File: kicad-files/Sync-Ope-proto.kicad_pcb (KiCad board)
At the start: 2 copper layers, 100 x 100 mm, 66 parts, among them J1 rca, J10 rca, J2 europower, J3 mono_jack_3.5mm, J4 mono_jack_3.5mm, J5 mono_jack_3.5mm, J6 rca, J7 barrel_jack, J8 diy_power_header, J9 rca, U1 AD8072, U2 74HC4538, U3 L7805, U4 L7905, U5 LT1251, U6 LM1881, U7 CD4053B

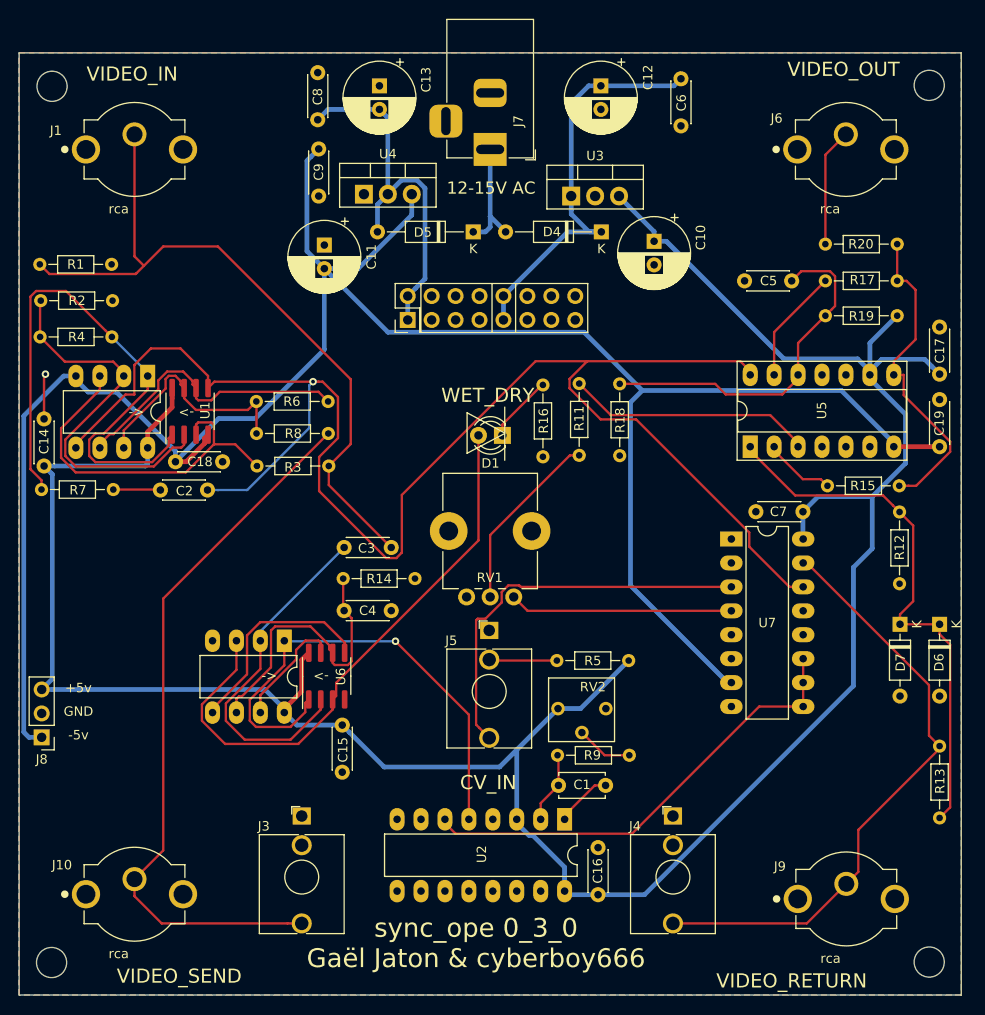
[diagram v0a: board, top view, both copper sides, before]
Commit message: working on v0.4.0
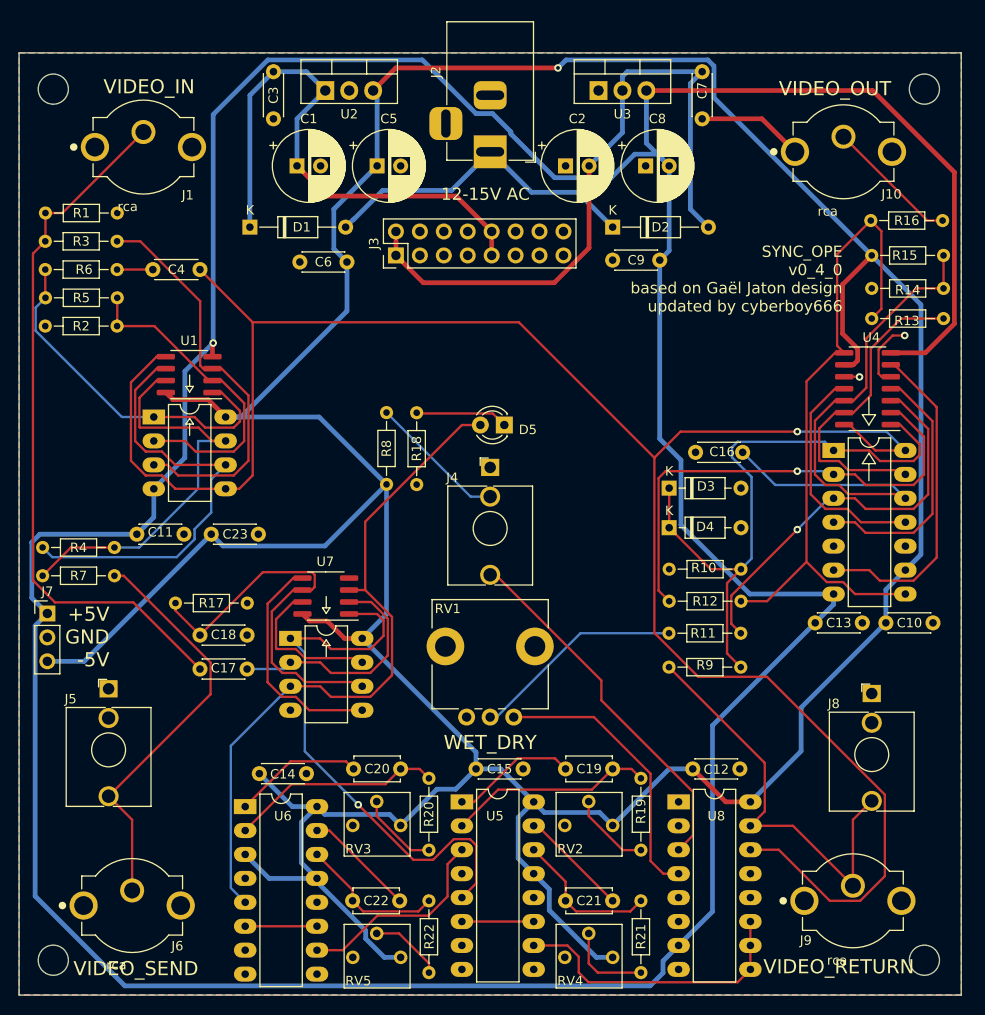
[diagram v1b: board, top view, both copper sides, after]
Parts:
- removed D6: zener_1.8v, Diode_THT:D_DO-35_SOD27_P7.62mm_Horizontal
- removed D7: schottky, Diode_THT:D_DO-35_SOD27_P7.62mm_Horizontal
- added C20: 0.1u, Capacitor_THT:C_Disc_D4.7mm_W2.5mm_P5.00mm, F.Cu at (135.5, 126.0)
- added C21: 1nf, Capacitor_THT:C_Disc_D4.7mm_W2.5mm_P5.00mm, F.Cu at (163.0, 140.0)
- added C22: 1uf, Capacitor_THT:C_Disc_D4.7mm_W2.5mm_P5.00mm, F.Cu at (140.4, 140.0)
- added C23: 0.1u, Capacitor_THT:C_Disc_D4.3mm_W1.9mm_P5.00mm, F.Cu at (120.4, 101.1)
- added D2: 1n4007, Diode_THT:D_DO-35_SOD27_P10.16mm_Horizontal, F.Cu at (163.0, 68.5)
- added D3: zener_1.8v, Diode_THT:D_DO-35_SOD27_P7.62mm_Horizontal, F.Cu at (169.0, 96.2)
- added R10: 470k, Resistor_THT:R_Axial_DIN0204_L3.6mm_D1.6mm_P7.62mm_Horizontal, F.Cu at (169.0, 104.8)
- added R21: 75k, Resistor_THT:R_Axial_DIN0204_L3.6mm_D1.6mm_P7.62mm_Horizontal, F.Cu at (166.0, 140.0)
- added R22: 22k, Resistor_THT:R_Axial_DIN0204_L3.6mm_D1.6mm_P7.62mm_Horizontal, F.Cu at (143.5, 140.0)
- added RV3: 10k_trim, lib_fp:tht_vertical_trim_3362, F.Cu at (140.5, 132.0)
- added RV4: 5k_trim, lib_fp:tht_vertical_trim_3362, F.Cu at (163.0, 146.0)
- added RV5: 10k_trim, lib_fp:tht_vertical_trim_3362, F.Cu at (140.5, 146.0)
- added U8: CD4053B, Package_DIP:DIP-16_W7.62mm_LongPads, F.Cu at (170.0, 129.5)
- C1: value 0.001u -> 220u; footprint Capacitor_THT:C_Disc_D4.7mm_W2.5mm_P5.00mm -> Capacitor_THT:CP_Radial_D7.5mm_P2.50mm
- C10, C11: value 100u -> 0.1u; footprint Capacitor_THT:CP_Radial_D7.5mm_P2.50mm -> Capacitor_THT:C_Disc_D4.3mm_W1.9mm_P5.00mm
- C12, C13: value 220u -> 0.1u; footprint Capacitor_THT:CP_Radial_D7.5mm_P2.50mm -> Capacitor_THT:C_Disc_D4.3mm_W1.9mm_P5.00mm
- C19: value 0.1u -> 1nf; footprint Capacitor_THT:C_Disc_D4.3mm_W1.9mm_P5.00mm -> Capacitor_THT:C_Disc_D4.7mm_W2.5mm_P5.00mm
- C2: value 0.1u -> 220u; footprint Capacitor_THT:C_Disc_D4.3mm_W1.9mm_P5.00mm -> Capacitor_THT:CP_Radial_D7.5mm_P2.50mm
- C3, C7: value 0.1u -> 0.33u
- C5: value 0.1u -> 100u; footprint Capacitor_THT:C_Disc_D4.3mm_W1.9mm_P5.00mm -> Capacitor_THT:CP_Radial_D7.5mm_P2.50mm
- C6: value 0.33u -> 0.1u
- C8: value 0.33u -> 100u; footprint Capacitor_THT:C_Disc_D4.3mm_W1.9mm_P5.00mm -> Capacitor_THT:CP_Radial_D7.5mm_P2.50mm
- D1: value LED -> 1n4007; footprint LED_THT:LED_D3.0mm -> Diode_THT:D_DO-35_SOD27_P10.16mm_Horizontal
- D4: value 1n4007 -> bat46; footprint Diode_THT:D_DO-35_SOD27_P10.16mm_Horizontal -> Diode_THT:D_DO-35_SOD27_P7.62mm_Horizontal
- D5: value 1n4007 -> LED; footprint Diode_THT:D_DO-35_SOD27_P10.16mm_Horizontal -> LED_THT:LED_D3.0mm
- J2: value europower -> barrel_jack; footprint Connector_PinHeader_2.54mm:PinHeader_2x08_P2.54mm_Vertical -> Connector_BarrelJack:BarrelJack_Horizontal
- J3: value mono_jack_3.5mm -> europower; footprint Connector_Audio:Jack_3.5mm_QingPu_WQP-PJ398SM_Vertical_CircularHoles -> Connector_PinHeader_2.54mm:PinHeader_2x08_P2.54mm_Vertical
- J7: value barrel_jack -> diy_power_header; footprint Connector_BarrelJack:BarrelJack_Horizontal -> Connector_PinHeader_2.54mm:PinHeader_1x03_P2.54mm_Vertical
- J8: value diy_power_header -> mono_jack_3.5mm; footprint Connector_PinHeader_2.54mm:PinHeader_1x03_P2.54mm_Vertical -> Connector_Audio:Jack_3.5mm_QingPu_WQP-PJ398SM_Vertical_CircularHoles
- R12: value 470k -> 1.5k
- R13: value 75 -> 1.5k
- R14: value 680k -> 10k
- R15: value 1.5k -> 47k
- R16: value 1k -> 75
- R17: value 1.5k -> 680k
- R18: value 10k -> 1k
- R19: value 47k -> 10k
- R20: value 75 -> 12k
- R5: value 39k -> 1.5k
- R6: value 1.5k -> 100
- R7: value 100 -> 75
- R8: value 75 -> 39k
- R9: value 10k -> 75
- RV1: value 10k -> 10k_pot; footprint Potentiometer_THT:Potentiometer_Alps_RK09K_Single_Vertical -> lib_fp:Potentiometer_Vertical_Large
- U2: value 74HC4538 -> L7805; footprint Package_DIP:DIP-16_W7.62mm_LongPads -> Package_TO_SOT_THT:TO-220-3_Vertical
- U3: value L7805 -> L7905
- U4: value L7905 -> LT1251; footprint Package_TO_SOT_THT:TO-220-3_Vertical -> lib_fp:DIP+SOIC_14
- U5: value LT1251 -> 74HC4538; footprint Package_DIP:DIP-14_W7.62mm_Socket_LongPads -> Package_DIP:DIP-16_W7.62mm_LongPads
- U6: value LM1881 -> 74HC4538; footprint lib_fp:DIP-SOIC-8 -> Package_DIP:DIP-16_W7.62mm_LongPads
- U7: value CD4053B -> LM1881; footprint Package_DIP:DIP-16_W7.62mm_LongPads -> lib_fp:DIP-SOIC-8
- moved J6 110.4 mm to (112.0, 140.5)
- moved J10 109.0 mm to (187.5, 60.5)
- moved J8 88.2 mm to (190.5, 118.0), turned to 0 degrees
- moved R17 83.9 mm to (116.6, 108.4), turned to 0 degrees
- moved U2 81.4 mm to (132.5, 54.0), turned to 0 degrees
- moved C17 79.9 mm to (124.2, 115.4), turned to 180 degrees
- moved C13 76.7 mm to (189.5, 110.5), turned to 180 degrees
- moved R20 75.4 mm to (143.5, 127.0), turned to 270 degrees
- moved C1 73.5 mm to (129.5, 62.0), turned to 0 degrees
- moved C12 73.2 mm to (171.5, 126.0), turned to 0 degrees
- moved R5 72.9 mm to (102.8, 76.0), turned to 0 degrees
- moved J7 68.1 mm to (103.0, 109.5), turned to 0 degrees
- moved R14 64.0 mm to (190.5, 75.0)
- moved J3 60.3 mm to (140.0, 71.5), turned to 90 degrees
- moved U4 59.6 mm to (190.5, 90.5)
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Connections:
- C1 pad 1: Net-(C1-Pad1) -> +12V
- C1 pad 2: Net-(C1-Pad2) -> GND
- C12 pad 1: +12V -> +5V
- C13 pad 2: -12V -> -5V
- C16 pad 1: +5V -> Net-(C16-Pad1)
- C17 pad 1: +5V -> Net-(C17-Pad1)
- C17 pad 2: GND -> /blanking/video_in
- C18 pad 1: GND -> Net-(C18-Pad1)
- C18 pad 2: -5V -> GND
- C19 pad 1: GND -> Net-(C19-Pad1)
- C19 pad 2: -5V -> Net-(C19-Pad2)
- C2 pad 1: /blanking/input_blank -> GND
- C2 pad 2: Net-(C2-Pad2) -> -12V
- C3 pad 1: Net-(C3-Pad1) -> +12V
- C3 pad 2: /blanking/video_in -> GND
- C4 pad 1: Net-(C4-Pad1) -> /blanking/input_blank
- C4 pad 2: GND -> Net-(C4-Pad2)
- C5 pad 1: Net-(C5-Pad1) -> +5V
- C6 pad 1: +12V -> +5V
- C7 pad 1: +5V -> GND
- C7 pad 2: GND -> -12V
- C8 pad 2: -12V -> -5V
- D1 pad 1: Net-(D1-Pad1) -> +12V
- D4 pad 1: +12V -> Net-(D3-Pad1)
- D4 pad 2: Net-(D4-Pad2) -> GND
- D5 pad 1: Net-(D4-Pad2) -> Net-(D5-Pad1)
- D5 pad 2: -12V -> Net-(D5-Pad2)
- J2 pad 1: -12V -> Net-(D1-Pad2)
- J2 pad 2: -12V -> GND
- J2 pad 3: GND -> Net-(J2-Pad3)
- J4 pad T: /blanking/return_blank -> /blanking/control_blank
- J5 pad T: /blanking/control_blank -> Net-(J5-PadT)
- J6 pad 1: Net-(J6-Pad1) -> Net-(J5-PadT)
- J7 pad 1: Net-(D4-Pad2) -> -5V
- J7 pad 3: Net-(J7-Pad3) -> +5V
- R12 pad 1: GND -> Net-(R12-Pad1)
- R12 pad 2: Net-(D6-Pad1) -> Net-(R12-Pad2)
- R13 pad 1: Net-(D6-Pad1) -> Net-(R12-Pad2)
- R13 pad 2: /blanking/return_blank -> Net-(R13-Pad2)
- R14 pad 1: Net-(C4-Pad1) -> GND
- R14 pad 2: GND -> Net-(C16-Pad1)
- R15 pad 1: Net-(R15-Pad1) -> +5V
- R15 pad 2: Net-(R15-Pad2) -> Net-(C16-Pad1)
- R16 pad 1: Net-(D1-Pad1) -> Net-(R12-Pad2)
- R16 pad 2: GND -> Net-(J10-Pad1)
- R17 pad 1: Net-(R15-Pad2) -> Net-(C18-Pad1)
- R17 pad 2: Net-(R17-Pad2) -> GND
- R18 pad 1: GND -> Net-(D5-Pad1)
- R18 pad 2: Net-(C5-Pad1) -> GND
- R19 pad 1: +5V -> Net-(C19-Pad2)
- R19 pad 2: Net-(C5-Pad1) -> Net-(R19-Pad2)
- R20 pad 1: Net-(R15-Pad2) -> Net-(C20-Pad2)
- R20 pad 2: Net-(J6-Pad1) -> Net-(R20-Pad2)
- R4 pad 2: Net-(R2-Pad1) -> Net-(R4-Pad2)
- R5 pad 1: +5V -> Net-(R5-Pad1)
- R5 pad 2: Net-(J5-PadTN) -> Net-(R2-Pad1)
- R6 pad 1: Net-(R6-Pad1) -> Net-(C4-Pad2)
- R6 pad 2: Net-(R6-Pad2) -> Net-(R5-Pad1)
- R7 pad 1: Net-(C2-Pad2) -> Net-(R4-Pad2)
- R7 pad 2: Net-(R4-Pad1) -> Net-(J5-PadT)
- R8 pad 1: Net-(R6-Pad2) -> +5V
- R8 pad 2: Net-(J10-Pad1) -> Net-(J4-PadTN)
- R9 pad 1: Net-(C1-Pad2) -> Net-(D3-Pad1)
- R9 pad 2: Net-(R9-Pad2) -> /blanking/return_blank
- RV2 pad 2: Net-(R9-Pad2) -> Net-(R19-Pad2)
- U1 pad 1: Net-(R4-Pad1) -> Net-(R5-Pad1)
- U1 pad 6: Net-(R6-Pad1) -> Net-(R4-Pad1)
- U1 pad 7: Net-(R6-Pad2) -> Net-(R4-Pad2)
- U2 pad 1: Net-(C1-Pad1) -> +12V
- U2 pad 2: Net-(C1-Pad2) -> GND
- U3 pad 1: +12V -> GND
- U3 pad 2: GND -> -12V
- U3 pad 3: +5V -> -5V
- U4 pad 1: GND -> Net-(D3-Pad1)
- U4 pad 2: -12V -> Net-(R12-Pad1)
- U4 pad 3: -5V -> Net-(R11-Pad1)
- U5 pad 1: Net-(D6-Pad1) -> Net-(C19-Pad1)
- U5 pad 10: GND -> c_blanking
- U5 pad 12: Net-(C5-Pad1) -> GND
- U5 pad 13: Net-(R17-Pad2) -> +5V
- U5 pad 14: /blanking/input_blank -> Net-(C21-Pad2)
- U5 pad 2: Net-(R15-Pad1) -> Net-(C19-Pad2)
- U5 pad 3: Net-(R11-Pad1) -> v_blanking
- U5 pad 4: Net-(U5-Pad4) -> GND
- U5 pad 5: GND -> Net-(U5-Pad5)
- U5 pad 6: Net-(U5-Pad6) -> Net-(U5-Pad11)
- U5 pad 7: -5V -> Net-(U5-Pad7)
- U5 pad 8: Net-(R15-Pad2) -> GND
- U5 pad 9: +5V -> Net-(U5-Pad9)
- U6 pad 1: Net-(U2-Pad5) -> Net-(C20-Pad1)
- U6 pad 2: Net-(C3-Pad1) -> Net-(C20-Pad2)
- U6 pad 3: Net-(D1-Pad2) -> +5V
- U6 pad 5: Net-(U6-Pad5) -> Net-(D5-Pad2)
- U6 pad 6: Net-(C4-Pad1) -> Net-(U6-Pad11)
- U6 pad 8: +5V -> GND
- U7 pad 1: Net-(U7-Pad1) -> Net-(U5-Pad5)
- U7 pad 2: GND -> Net-(C17-Pad1)
- U7 pad 3: /blanking/control_blank -> Net-(D5-Pad2)
- U7 pad 4: /blanking/control_pulse -> GND
- U7 pad 5: GND -> Net-(U7-Pad5)
- U7 pad 6: GND -> Net-(C18-Pad1)
- U7 pad 7: -5V -> Net-(U7-Pad7)
- U7 pad 8: GND -> +5V
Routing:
- net -5V: track 230.3 -> 404.3 mm, vias 0 -> 1
- net +5V: track 279.3 -> 423.1 mm, vias 0 -> 1
- net Net-(D5-Pad2): track 0.00 -> 74.0 mm
- net Net-(R12-Pad2): track 0.00 -> 72.1 mm
- net Net-(D3-Pad1): track 0.00 -> 65.9 mm
- net Net-(J10-Pad1): track 76.6 -> 14.2 mm
- net Net-(C16-Pad1): track 0.00 -> 61.7 mm
- net Net-(U5-Pad5): track 0.00 -> 59.4 mm, vias 0 -> 1
- net Net-(D6-Pad1): track 57.7 -> 0.00 mm
- net Net-(U2-Pad5): track 52.3 -> 0.00 mm, vias 1 -> 0
- net Net-(R12-Pad1): track 0.00 -> 51.7 mm, vias 0 -> 1
- net Net-(U2-Pad6): track 49.6 -> 0.00 mm
- net /blanking/input_blank: track 166.9 -> 213.3 mm
- net Net-(R4-Pad2): track 0.00 -> 44.7 mm
- net Net-(J5-PadT): track 0.00 -> 43.7 mm
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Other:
- board text added: "+5V GND -5V"
- board text added: "SYNC_OPE v0_4_0 based on Gaël Jaton design updated by cyberboy666"
- board text removed: "+5v"
- board text removed: "-5v"
- board text removed: "->"
- board text removed: "CV_IN"
- board text removed: "GND"
- board text removed: "sync_ope 0_3_0 Gaël Jaton & cyberboy666"
